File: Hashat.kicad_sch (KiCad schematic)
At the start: 0 parts

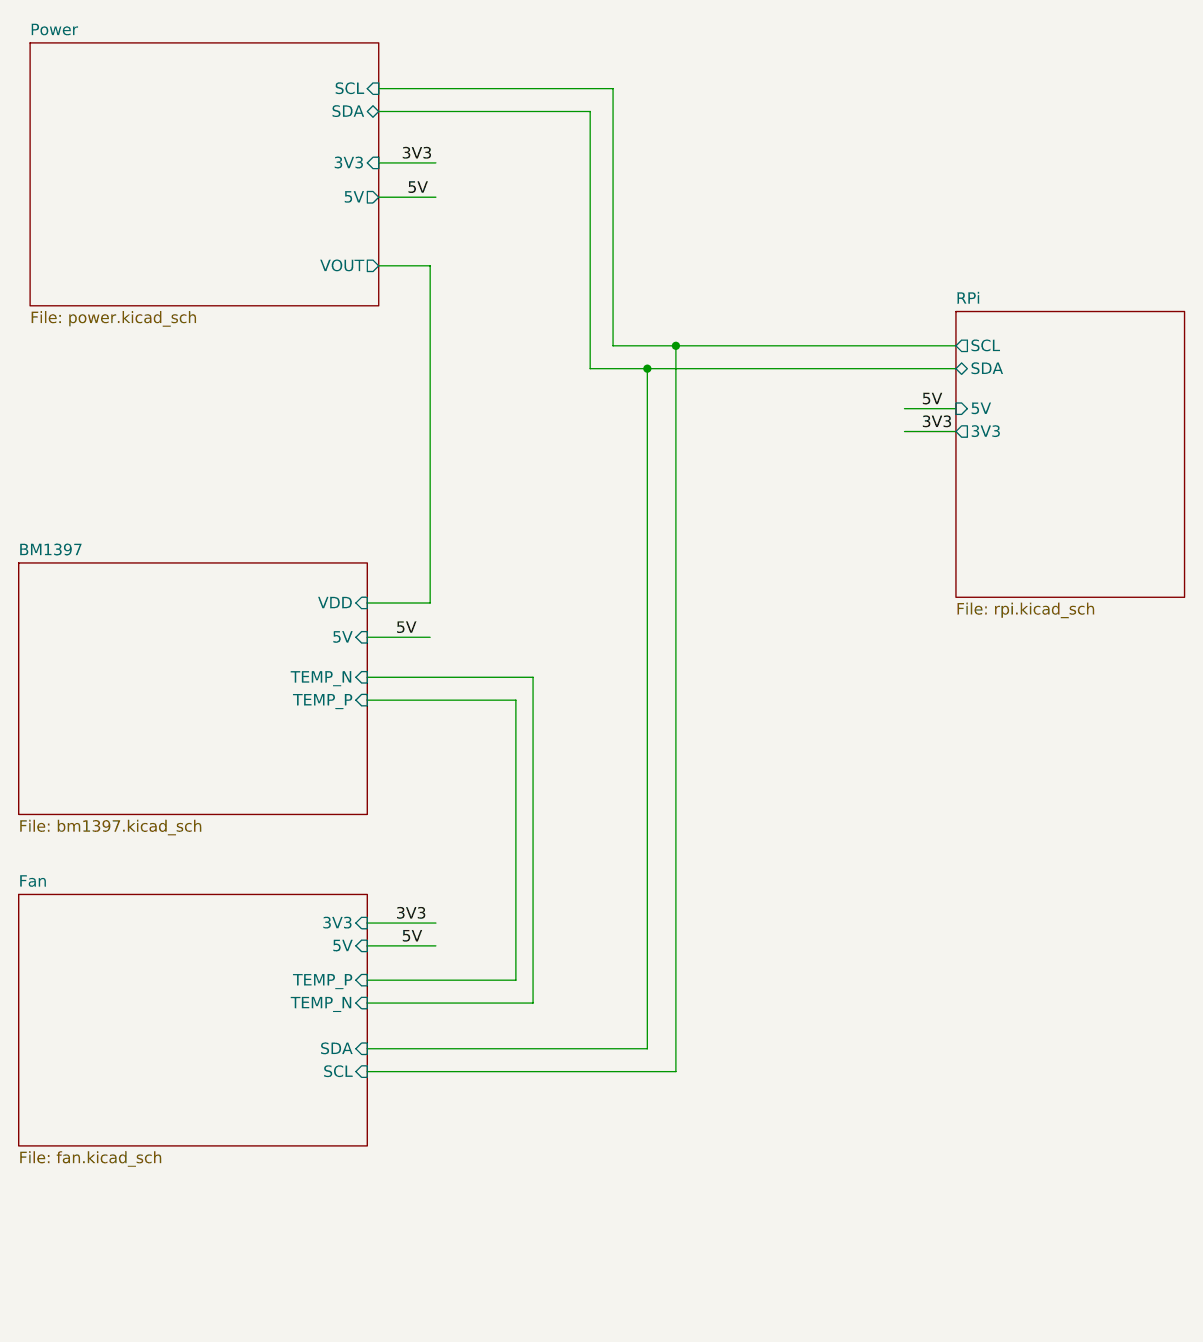
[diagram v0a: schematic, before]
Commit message: more schematic
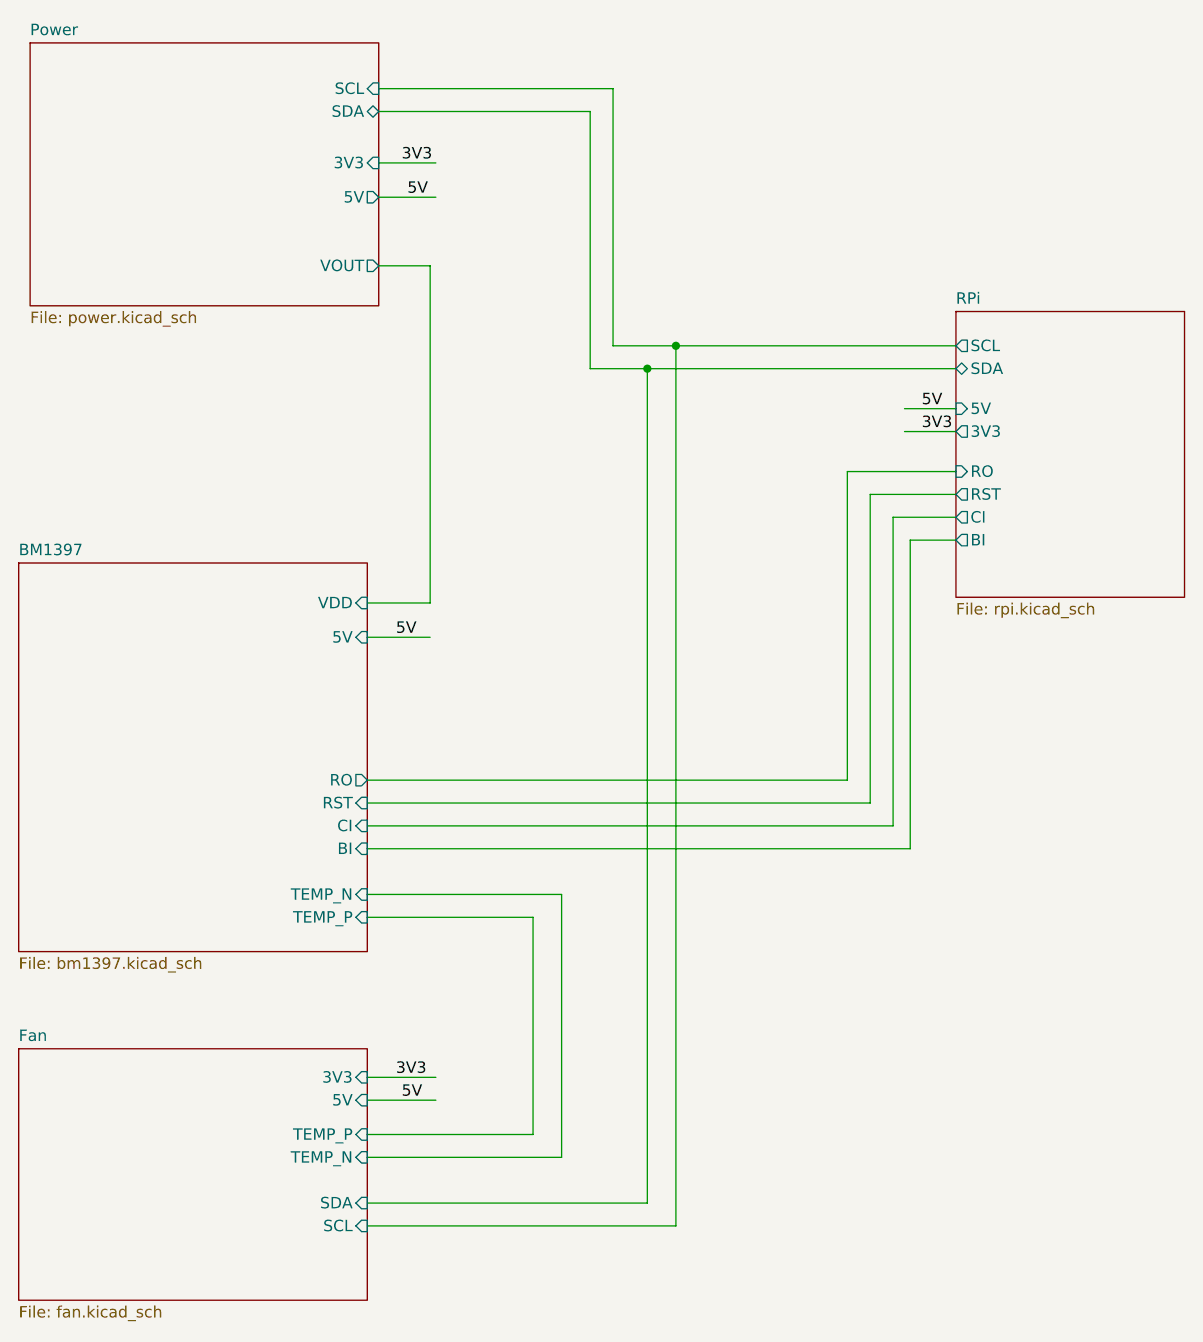
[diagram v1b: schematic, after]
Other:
- sheet BM1397 ports: added BI, CI, RO, RST; removed none
- sheet RPi ports: added BI, CI, RO, RST; removed none
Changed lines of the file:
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@@
+    (stroke (width 0) (type default))
+  )
+  (wire (pts (xy 96.52 127) (xy 154.94 127))
     (stroke (width 0) (type default))
   )
@@
     (stroke (width 0) (type default))
   )
+  (wire (pts (xy 96.52 121.92) (xy 149.86 121.92))
+    (stroke (width 0) (type default))
+  )
+  (wire (pts (xy 152.4 90.17) (xy 152.4 124.46))
+    (stroke (width 0) (type default))
+  )
   (wire (pts (xy 97.79 64.77) (xy 103.505 64.77))
     (stroke (width 0) (type default))
@@
     (stroke (width 0) (type default))
   )
-  (wire (pts (xy 96.52 144.145) (xy 113.03 144.145))
+  (wire (pts (xy 96.52 161.29) (xy 114.935 161.29))
     (stroke (width 0) (type default))
   )
@@
     (stroke (width 0) (type default))
   )
+  (wire (pts (xy 154.94 92.71) (xy 161.925 92.71))
+    (stroke (width 0) (type default))
+  )
   (wire (pts (xy 156.21 80.645) (xy 161.925 80.645))
     (stroke (width 0) (type default))
   )
-  (wire (pts (xy 113.03 144.145) (xy 113.03 113.03))
+  (wire (pts (xy 114.935 161.29) (xy 114.935 137.16))
     (stroke (width 0) (type default))
   )
@@
     (stroke (width 0) (type default))
   )
-  (wire (pts (xy 127.635 151.765) (xy 127.635 76.2))
-    (stroke (width 0) (type default))
-  )
-  (wire (pts (xy 96.52 151.765) (xy 127.635 151.765))
+  (wire (pts (xy 127.635 168.91) (xy 127.635 76.2))
+    (stroke (width 0) (type default))
+  )
+  (wire (pts (xy 96.52 168.91) (xy 127.635 168.91))
     (stroke (width 0) (type default))
   )
@@
     (stroke (width 0) (type default))
   )
-  (wire (pts (xy 113.03 113.03) (xy 96.52 113.03))
-    (stroke (width 0) (type default))
-  )
-  (wire (pts (xy 96.52 154.305) (xy 130.81 154.305))
-    (stroke (width 0) (type default))
-  )
-  (wire (pts (xy 114.935 110.49) (xy 114.935 146.685))
+  (wire (pts (xy 114.935 137.16) (xy 96.52 137.16))
+    (stroke (width 0) (type default))
+  )
+  (wire (pts (xy 96.52 171.45) (xy 130.81 171.45))
+    (stroke (width 0) (type default))
+  )
+  (wire (pts (xy 118.11 134.62) (xy 118.11 163.83))
+    (stroke (width 0) (type default))
+  )
+  (wire (pts (xy 161.925 95.25) (xy 156.845 95.25))
+    (stroke (width 0) (type default))
+  )
+  (wire (pts (xy 161.925 90.17) (xy 152.4 90.17))
+    (stroke (width 0) (type default))
+  )
+  (wire (pts (xy 154.94 127) (xy 154.94 92.71))
     (stroke (width 0) (type default))
   )
@@
     (stroke (width 0) (type default))
   )
-  (wire (pts (xy 96.52 110.49) (xy 114.935 110.49))
+  (wire (pts (xy 96.52 134.62) (xy 118.11 134.62))
     (stroke (width 0) (type default))
   )
@@
     (stroke (width 0) (type default))
   )
-  (wire (pts (xy 114.935 146.685) (xy 96.52 146.685))
-    (stroke (width 0) (type default))
-  )
-  (wire (pts (xy 130.81 154.305) (xy 130.81 73.66))
+  (wire (pts (xy 149.86 87.63) (xy 161.925 87.63))
+    (stroke (width 0) (type default))
+  )
+  (wire (pts (xy 118.11 163.83) (xy 96.52 163.83))
+    (stroke (width 0) (type default))
+  )
+  (wire (pts (xy 156.845 129.54) (xy 96.52 129.54))
+    (stroke (width 0) (type default))
+  )
+  (wire (pts (xy 130.81 171.45) (xy 130.81 73.66))
+    (stroke (width 0) (type default))
+  )
+  (wire (pts (xy 152.4 124.46) (xy 96.52 124.46))
     (stroke (width 0) (type default))
   )
@@
     (stroke (width 0) (type default))
   )
-  (wire (pts (xy 96.52 137.795) (xy 104.14 137.795))
-    (stroke (width 0) (type default))
-  )
-  (wire (pts (xy 96.52 140.335) (xy 104.14 140.335))
+  (wire (pts (xy 96.52 154.94) (xy 104.14 154.94))
+    (stroke (width 0) (type default))
+  )
+  (wire (pts (xy 149.86 121.92) (xy 149.86 87.63))
+    (stroke (width 0) (type default))
+  )
+  (wire (pts (xy 156.845 95.25) (xy 156.845 129.54))
+    (stroke (width 0) (type default))
+  )
+  (wire (pts (xy 96.52 157.48) (xy 104.14 157.48))
     (stroke (width 0) (type default))
   )
@@
     (effects (font (size 1.27 1.27)) (justify left bottom))
   )
-  (label "5V" (at 100.33 140.335 0) (fields_autoplaced)
+  (label "5V" (at 100.33 157.48 0) (fields_autoplaced)
     (effects (font (size 1.27 1.27)) (justify left bottom))
   )
@@
     (effects (font (size 1.27 1.27)) (justify left bottom))
   )
-  (label "3V3" (at 99.695 137.795 0) (fields_autoplaced)
+  (label "3V3" (at 99.695 154.94 0) (fields_autoplaced)
     (effects (font (size 1.27 1.27)) (justify left bottom))
   )
@@
     )
     (pin "3V3" output (at 161.925 83.185 180)
+      (effects (font (size 1.27 1.27)) (justify left))
+    )
+    (pin "CI" output (at 161.925 92.71 180)
+      (effects (font (size 1.27 1.27)) (justify left))
+    )
+    (pin "RO" input (at 161.925 87.63 180)
+      (effects (font (size 1.27 1.27)) (justify left))
+    )
+    (pin "BI" output (at 161.925 95.25 180)
+      (effects (font (size 1.27 1.27)) (justify left))
+    )
+    (pin "RST" output (at 161.925 90.17 180)
       (effects (font (size 1.27 1.27)) (justify left))
     )
@@
     )
   )
-  (sheet (at 57.785 97.79) (size 38.735 27.94) (fields_autoplaced)
+  (sheet (at 57.785 97.79) (size 38.735 43.18) (fields_autoplaced)
     (stroke (width 0.1524) (type solid))
     (fill (color 255 255 194 1.0000))
@@
       (effects (font (size 1.27 1.27)) (justify left bottom))
     )
-    (property "Sheetfile" "bm1397.kicad_sch" (at 57.785 126.3146 0)
+    (property "Sheetfile" "bm1397.kicad_sch" (at 57.785 141.5546 0)
       (effects (font (size 1.27 1.27)) (justify left top))
     )
@@
       (effects (font (size 1.27 1.27)) (justify right))
     )
-    (pin "TEMP_N" input (at 96.52 110.49 0)
-      (effects (font (size 1.27 1.27)) (justify right))
-    )
-    (pin "TEMP_P" input (at 96.52 113.03 0)
+    (pin "TEMP_N" input (at 96.52 134.62 0)
+      (effects (font (size 1.27 1.27)) (justify right))
+    )
+    (pin "TEMP_P" input (at 96.52 137.16 0)
+      (effects (font (size 1.27 1.27)) (justify right))
+    )
+    (pin "RO" output (at 96.52 121.92 0)
+      (effects (font (size 1.27 1.27)) (justify right))
+    )
+    (pin "RST" input (at 96.52 124.46 0)
+      (effects (font (size 1.27 1.27)) (justify right))
+    )
+    (pin "CI" input (at 96.52 127 0)
+      (effects (font (size 1.27 1.27)) (justify right))
+    )
+    (pin "BI" input (at 96.52 129.54 0)
       (effects (font (size 1.27 1.27)) (justify right))
     )
@@
     )
   )
-  (sheet (at 57.785 134.62) (size 38.735 27.94) (fields_autoplaced)
-    (stroke (width 0.1524) (type solid))
-    (fill (color 255 255 194 1.0000))
-    (property "Sheetname" "Fan" (at 57.785 133.9084 0)
-      (effects (font (size 1.27 1.27)) (justify left bottom))
-    )
-    (property "Sheetfile" "fan.kicad_sch" (at 57.785 163.1446 0)
-      (effects (font (size 1.27 1.27)) (justify left top))
-    )
-    (pin "5V" input (at 96.52 140.335 0)
-      (effects (font (size 1.27 1.27)) (justify right))
-    )
-    (pin "TEMP_P" input (at 96.52 144.145 0)
-      (effects (font (size 1.27 1.27)) (justify right))
-    )
-    (pin "TEMP_N" input (at 96.52 146.685 0)
-      (effects (font (size 1.27 1.27)) (justify right))
-    )
-    (pin "3V3" input (at 96.52 137.795 0)
-      (effects (font (size 1.27 1.27)) (justify right))
-    )
-    (pin "SDA" input (at 96.52 151.765 0)
-      (effects (font (size 1.27 1.27)) (justify right))
-    )
-    (pin "SCL" input (at 96.52 154.305 0)
-      (effects (font (size 1.27 1.27)) (justify right))
-    )
+  (sheet (at 57.785 151.765) (size 38.735 27.94) (fields_autoplaced)
+    (stroke (width 0.1524) (type solid))
+    (fill (color 255 255 194 1.0000))
+    (property "Sheetname" "Fan" (at 57.785 151.0534 0)
+      (effects (font (size 1.27 1.27)) (justify left bottom))
+    )
+    (property "Sheetfile" "fan.kicad_sch" (at 57.785 180.2896 0)
+      (effects (font (size 1.27 1.27)) (justify left top))
+    )
+    (pin "5V" input (at 96.52 157.48 0)
+      (effects (font (size 1.27 1.27)) (justify right))
+    )
+    (pin "TEMP_P" input (at 96.52 161.29 0)
+      (effects (font (size 1.27 1.27)) (justify right))
+    )
+    (pin "TEMP_N" input (at 96.52 163.83 0)
+      (effects (font (size 1.27 1.27)) (justify right))
+    )
+    (pin "3V3" input (at 96.52 154.94 0)
+      (effects (font (size 1.27 1.27)) (justify right))
+    )
+    (pin "SDA" input (at 96.52 168.91 0)
+      (effects (font (size 1.27 1.27)) (justify right))
+    )
+    (pin "SCL" input (at 96.52 171.45 0)
+      (effects (font (size 1.27 1.27)) (justify right))
+    )
